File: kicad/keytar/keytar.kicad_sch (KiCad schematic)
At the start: 28 parts, among them J1 , J2 USB_B, J3 AudioJack2, J4 Conn_01x04, J5 USB_A, J6 Mini-DIN-6-Shielded, J7 Conn_01x04, Q1 BSS138, Q2 BSS138, U1 Pico, U2 MCP73831-2-OT

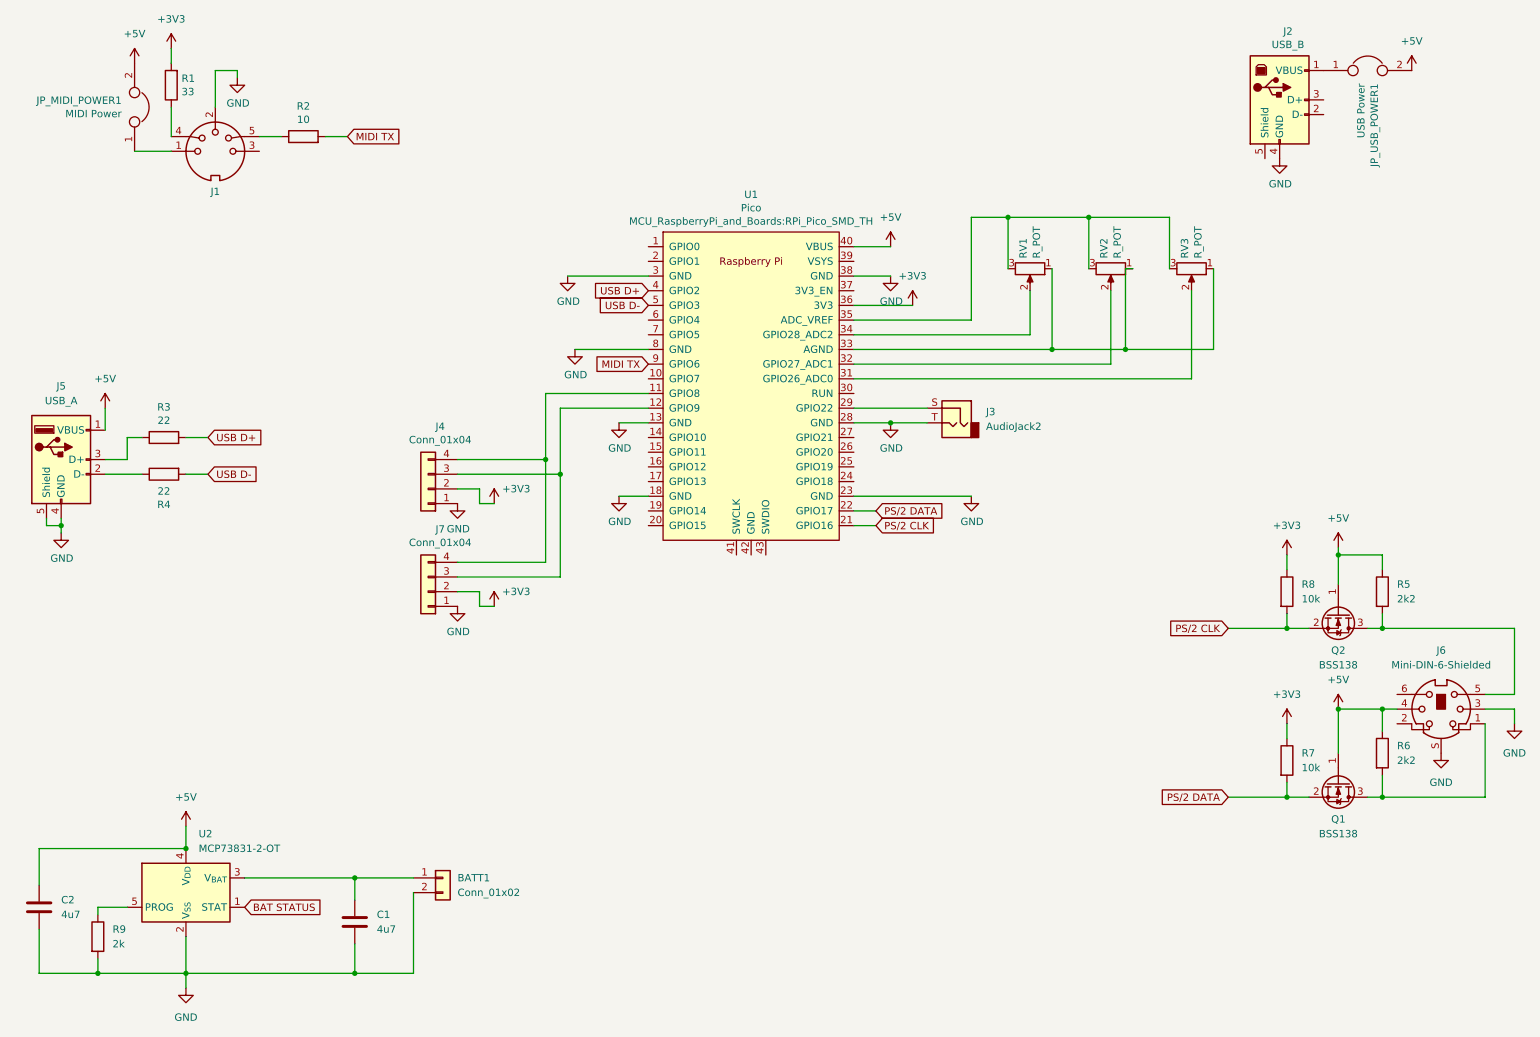
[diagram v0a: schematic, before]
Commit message: route board
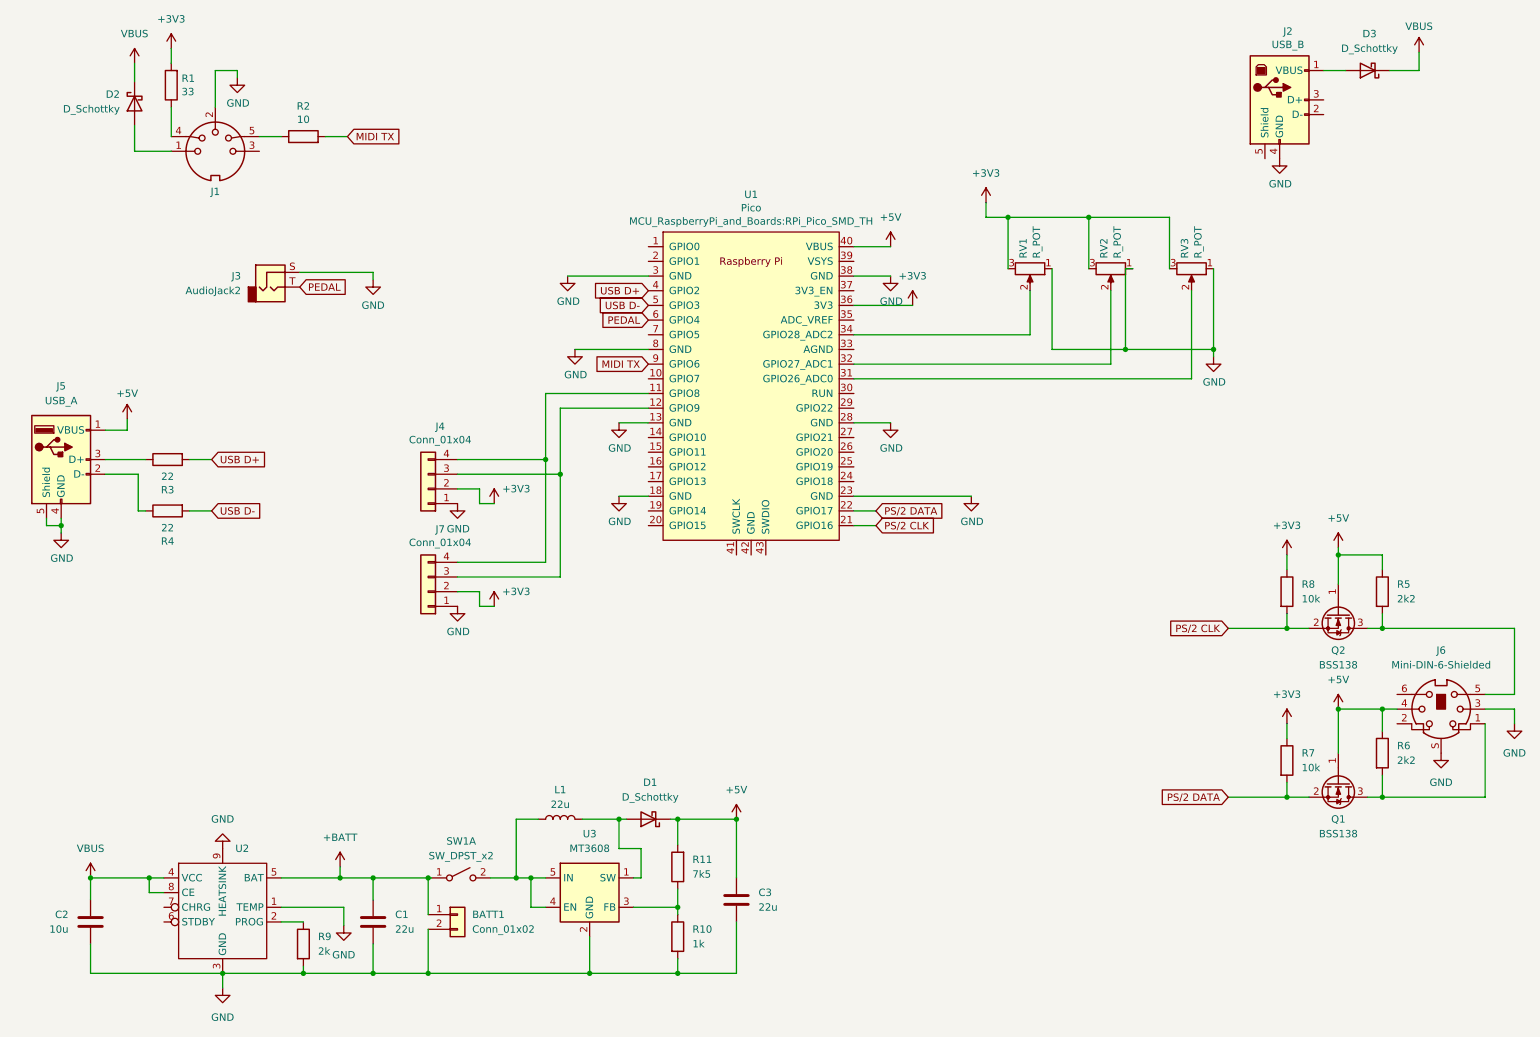
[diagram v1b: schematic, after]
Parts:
- removed JP_MIDI_POWER1: MIDI Power, Connector_PinHeader_2.54mm:PinHeader_1x02_P2.54mm_Vertical, symbol keytar-rescue:Jumper-Device
- removed JP_USB_POWER1: USB Power, Connector_PinHeader_2.54mm:PinHeader_1x02_P2.54mm_Vertical, symbol keytar-rescue:Jumper-Device
- removed U2: MCP73831-2-OT, Package_TO_SOT_SMD:SOT-23-5, symbol Battery_Management:MCP73831-2-OT
- added C3: 22u, Capacitor_SMD:C_1206_3216Metric_Pad1.33x1.80mm_HandSolder, symbol Device:C
- added D1, D2, D3: D_Schottky, Diode_SMD:D_SMA, symbol Device:D_Schottky
- added L1: 22u, Inductor_SMD:L_Bourns-SRN4018, symbol Device:L
- added R10: 1k, Resistor_SMD:R_1206_3216Metric_Pad1.30x1.75mm_HandSolder, symbol Device:R
- added R11: 7k5, Resistor_SMD:R_1206_3216Metric_Pad1.30x1.75mm_HandSolder, symbol Device:R
- added SW1: SW_DPST_x2, symbol Switch:SW_DPST_x2
- added U2: ~, Package_SO:HSOP-8-1EP_3.9x4.9mm_P1.27mm_EP2.3x2.3mm_ThermalVias, symbol keytar-parts:TP4056
- added U3: MT3608, Package_TO_SOT_SMD:SOT-23-6, symbol Regulator_Switching:MT3608
- C1: value 4u7 -> 22u
- C2: value 4u7 -> 10u
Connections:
- net +3V3: now also RV1.3, RV2.3, RV3.3
- net +5V: now also C3.1, D1.1 (K), R11.2; no longer C2.1
- net GND: now also J3.S, RV1.1, RV2.1, RV3.1, C3.2, R10.2, U2.1 (TEMP), U2.3 (GND), U2.9 (HEATSINK), U3.2 (GND); no longer J3.T
- net at U1.29 (GPIO22): no longer J3.S
- net PEDAL: now reaches U1.6 (GPIO4)
- net PEDAL: now also J3.T
- net at J2.1 (VBUS): now also D3.2 (A)
- net at J1.1: now also D2.2 (A)
- net +BATT: now reaches BATT1.1 (Pin_1), C1.1
- net +BATT: now also SW1.1 (A), U2.5 (BAT)
- net at R9.1: now also U2.2 (PROG)
- new net: L1.1, SW1.2 (B), U3.4 (EN), U3.5 (IN)
- new net: D1.2 (A), L1.2, U3.1 (SW)
- new net: R10.1, R11.1, U3.3 (FB)
- new net VBUS: C2.1, D2.1 (K), D3.1 (K), U2.4 (VCC), U2.8 (CE)
- now unconnected: U1.33 (AGND), U1.35 (ADC_VREF)
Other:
- moved on the sheet: BATT1, C1, C2, J3, R3, R4

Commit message: improve pcb
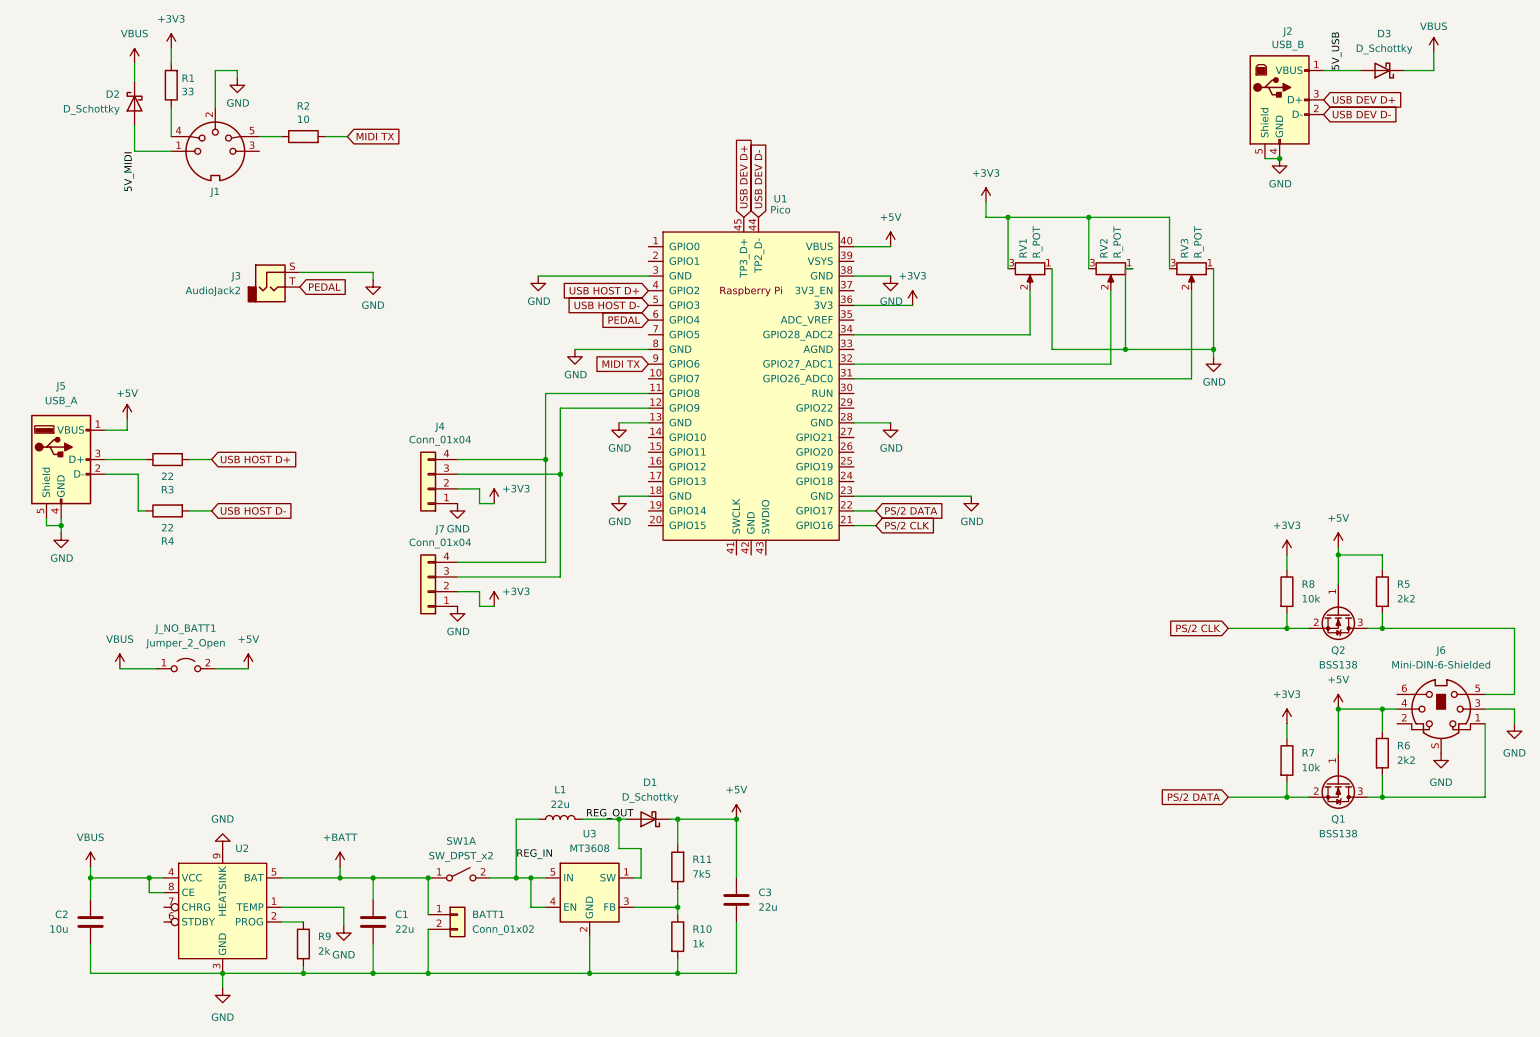
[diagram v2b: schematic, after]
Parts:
- added J_NO_BATT1: Jumper_2_Open, Jumper:SolderJumper-2_P1.3mm_Open_RoundedPad1.0x1.5mm, symbol Jumper:Jumper_2_Open
- SW1: footprint (none) -> Connector_JST:JST_XH_B3B-XH-A_1x03_P2.50mm_Vertical
- U1: footprint MCU_RaspberryPi_and_Boards:RPi_Pico_SMD_TH -> keyar-parts:RPi_Pico_debug_hole_USB_SMD_TH; symbol keytar-rescue:Pico-MCU_RaspberryPi_and_Boards -> keytar-parts:Pico_USB
- U2: footprint Package_SO:HSOP-8-1EP_3.9x4.9mm_P1.27mm_EP2.3x2.3mm_ThermalVias -> Package_SO:HSOP-8-1EP_3.9x4.9mm_P1.27mm_EP2.3x2.3mm
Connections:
- net +5V: now also J_NO_BATT1.2 (B)
- net GND: now also J2.5 (Shield)
- net VBUS: now also J_NO_BATT1.1 (A)
- net 5V_USB: now reaches D3.2 (A), J2.1 (VBUS)
- net USB DEV D-: now reaches J2.2 (D-)
- net USB DEV D-: now also U1.44 (TP2_D-)
- net USB DEV D+: now reaches J2.3 (D+)
- net USB DEV D+: now also U1.45 (TP3_D+)
- net 5V_MIDI: now reaches D2.2 (A), J1.1
- net REG_IN: now reaches L1.1, SW1.2 (B), U3.4 (EN), U3.5 (IN)
- net REG_OUT: now reaches D1.2 (A), L1.2, U3.1 (SW)
- net USB D+ renamed USB HOST D+
- net USB D- renamed USB HOST D-
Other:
- moved on the sheet: D3
